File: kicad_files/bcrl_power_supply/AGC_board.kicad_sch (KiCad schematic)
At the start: 1 part, among them J59 Conn_01x04_Pin

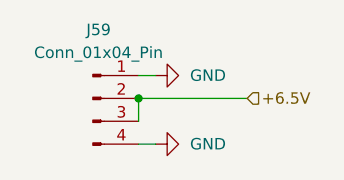
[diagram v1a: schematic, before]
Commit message: schematic done
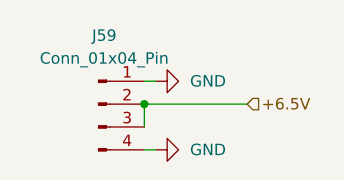
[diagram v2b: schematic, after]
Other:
- moved on the sheet: J59
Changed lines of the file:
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@@
 	(paper "A4")
 	(junction
-		(at 37.465 45.085)
+		(at 38.1 45.72)
 		(diameter 0)
 		(color 0 0 0 0)
@@
 	(wire
 		(pts
-			(xy 49.53 45.085) (xy 37.465 45.085)
-		)
-		(stroke
-			(width 0)
-			(type default)
-		)
-	)
-	(wire
-		(pts
-			(xy 39.37 50.165) (xy 37.465 50.165)
-		)
-		(stroke
-			(width 0)
-			(type default)
-		)
-	)
-	(wire
-		(pts
-			(xy 39.37 42.545) (xy 37.465 42.545)
-		)
-		(stroke
-			(width 0)
-			(type default)
-		)
-	)
-	(wire
-		(pts
-			(xy 37.465 45.085) (xy 37.465 47.625)
+			(xy 49.53 45.72) (xy 38.1 45.72)
+		)
+		(stroke
+			(width 0)
+			(type default)
+		)
+	)
+	(wire
+		(pts
+			(xy 39.37 50.8) (xy 38.1 50.8)
+		)
+		(stroke
+			(width 0)
+			(type default)
+		)
+	)
+	(wire
+		(pts
+			(xy 39.37 43.18) (xy 38.1 43.18)
+		)
+		(stroke
+			(width 0)
+			(type default)
+		)
+	)
+	(wire
+		(pts
+			(xy 38.1 45.72) (xy 38.1 48.26)
 		)
 		(stroke
@@
 	(hierarchical_label "+6.5V"
 		(shape input)
-		(at 49.53 45.085 0)
+		(at 49.53 45.72 0)
 		(fields_autoplaced yes)
 		(effects
@@
 	(symbol
 		(lib_id "Connector:Conn_01x04_Pin")
-		(at 32.385 45.085 0)
+		(at 33.02 45.72 0)
 		(unit 1)
 		(exclude_from_sim no)
@@
 		(fields_autoplaced yes)
 		(property "Reference" "J59"
-			(at 33.02 37.465 0)
+			(at 33.655 38.1 0)
 			(effects
 				(font
@@
 		)
 		(property "Value" "Conn_01x04_Pin"
-			(at 33.02 40.005 0)
+			(at 33.655 40.64 0)
 			(effects
 				(font
@@
 		)
 		(property "Footprint" "Connector_PinHeader_2.54mm:PinHeader_1x04_P2.54mm_Vertical"
-			(at 32.385 45.085 0)
+			(at 33.02 45.72 0)
 			(effects
 				(font
@@
 		)
 		(property "Datasheet" "~"
-			(at 32.385 45.085 0)
+			(at 33.02 45.72 0)
 			(effects
 				(font
@@
 		)
 		(property "Description" ""
-			(at 32.385 45.085 0)
+			(at 33.02 45.72 0)
 			(effects
 				(font
@@
 	(symbol
 		(lib_id "power:GND")
-		(at 39.37 50.165 90)
+		(at 39.37 50.8 90)
 		(unit 1)
 		(exclude_from_sim no)
@@
 		(fields_autoplaced yes)
 		(property "Reference" "#PWR0196"
-			(at 45.72 50.165 0)
+			(at 45.72 50.8 0)
 			(effects
 				(font
@@
 		)
 		(property "Value" "GND"
-			(at 43.18 50.165 90)
+			(at 43.18 50.8 90)
 			(effects
 				(font
@@
 		)
 		(property "Footprint" ""
-			(at 39.37 50.165 0)
+			(at 39.37 50.8 0)
 			(effects
 				(font
@@
 		)
 		(property "Datasheet" ""
-			(at 39.37 50.165 0)
+			(at 39.37 50.8 0)
 			(effects
 				(font
@@
 		)
 		(property "Description" ""
-			(at 39.37 50.165 0)
+			(at 39.37 50.8 0)
 			(effects
 				(font
@@
 	(symbol
 		(lib_id "power:GND")
-		(at 39.37 42.545 90)
+		(at 39.37 43.18 90)
 		(unit 1)
 		(exclude_from_sim no)
@@
 		(fields_autoplaced yes)
 		(property "Reference" "#PWR0195"
-			(at 45.72 42.545 0)
+			(at 45.72 43.18 0)
 			(effects
 				(font
@@
 		)
 		(property "Value" "GND"
-			(at 43.18 42.545 90)
+			(at 43.18 43.18 90)
 			(effects
 				(font
@@
 		)
 		(property "Footprint" ""
-			(at 39.37 42.545 0)
+			(at 39.37 43.18 0)
 			(effects
 				(font
@@
 		)
 		(property "Datasheet" ""
-			(at 39.37 42.545 0)
+			(at 39.37 43.18 0)
 			(effects
 				(font
@@
 		)
 		(property "Description" ""
-			(at 39.37 42.545 0)
-			(effects
-				(font
+			(at 39.37 43.18 0)
+			(effects
+				(font
